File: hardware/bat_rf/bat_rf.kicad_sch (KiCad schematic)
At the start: 54 parts, among them J1 USB_C_Receptacle_PowerOnly_6P, J2 Conn_01x02, J3 burningPort, Q1 NMOS, SW1 SW_DPDT_x2, SW2 RESET, U1 TPS5430DDA, U2 AMS1117, U3 ESP8684-WROOM-02UC, U4 CS5090E

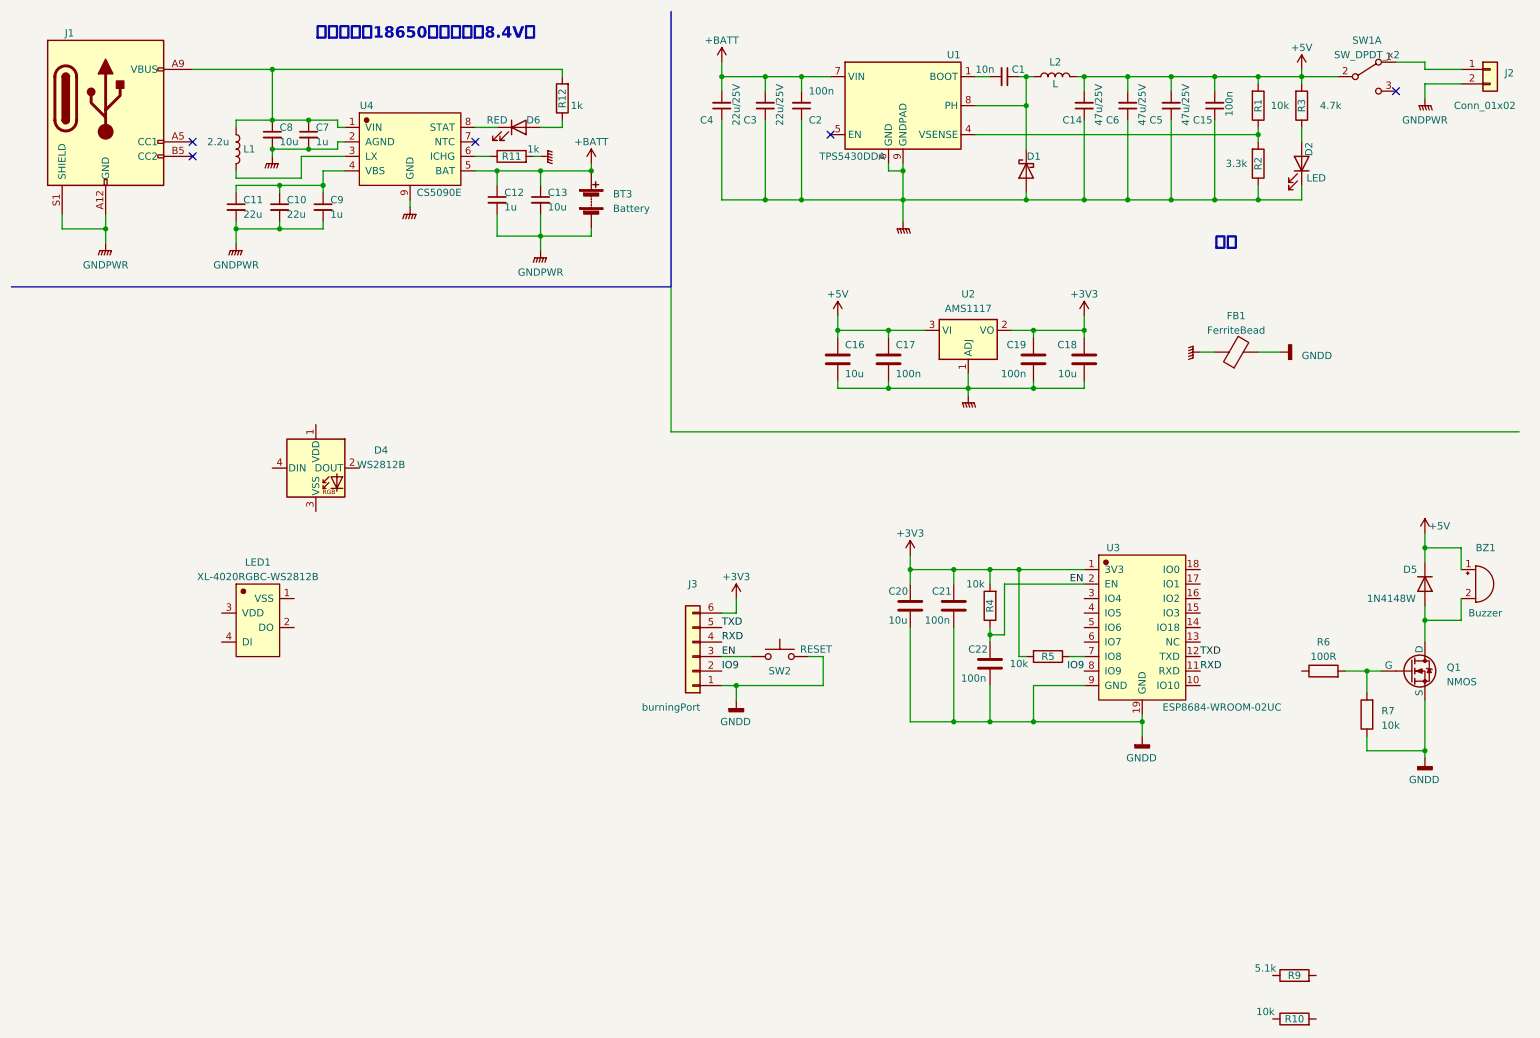
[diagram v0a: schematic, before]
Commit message: hardware update
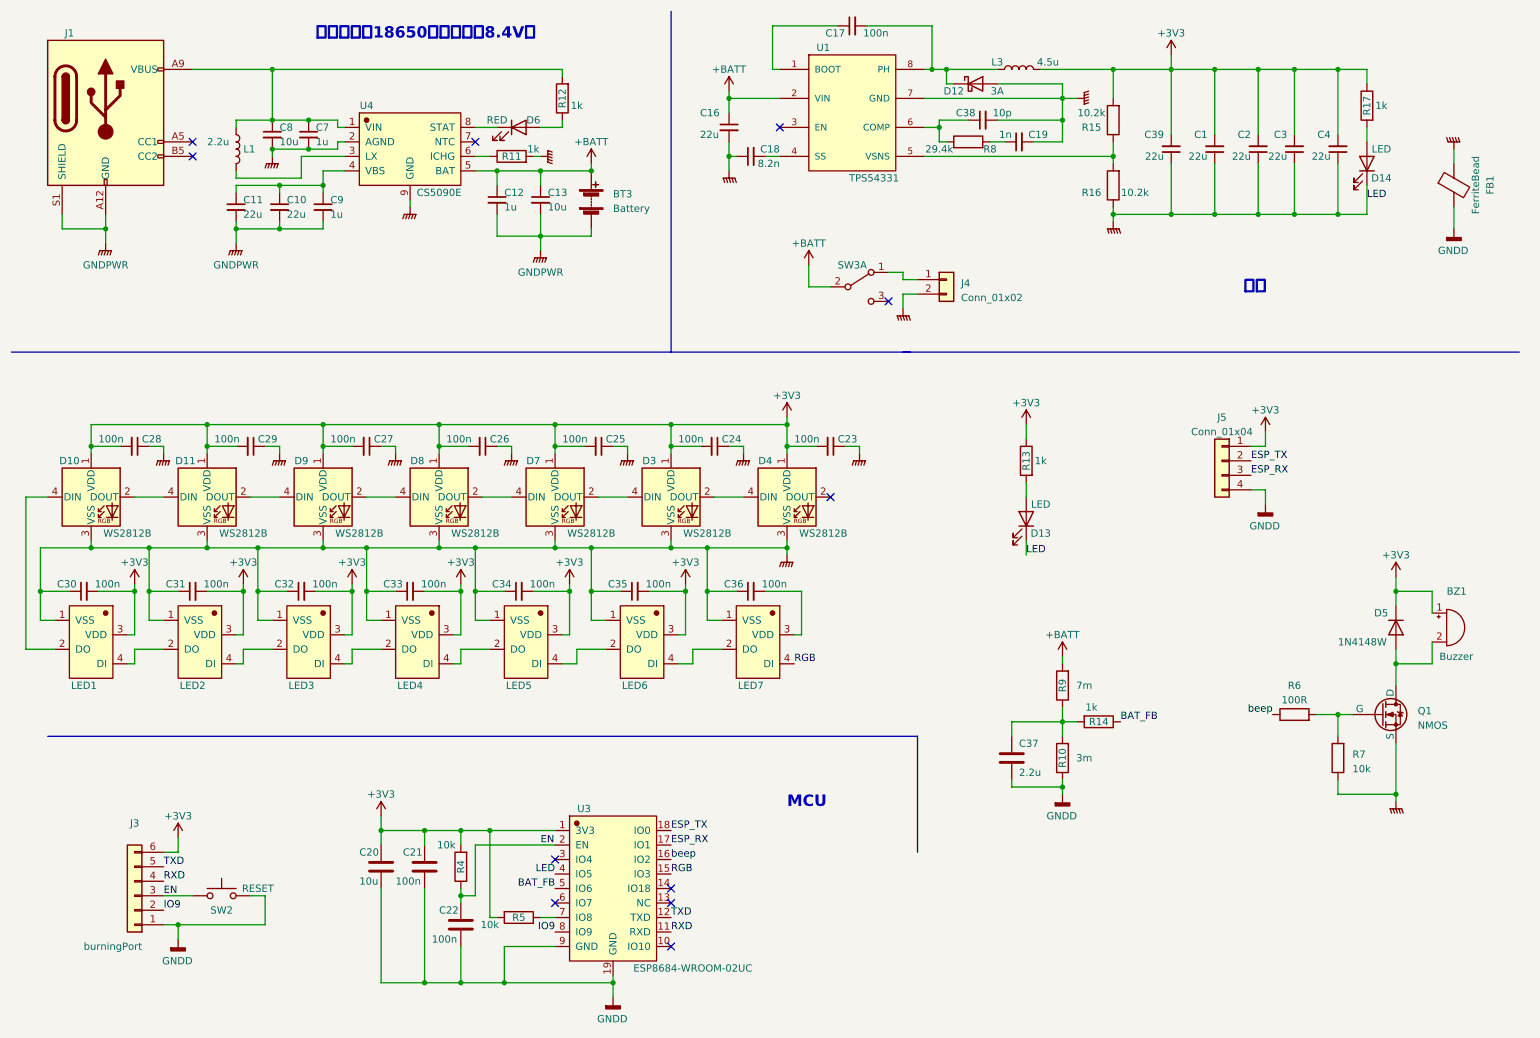
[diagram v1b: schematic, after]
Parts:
- removed C14, C5, C6: 47u/25V, symbol Device:C_Small
- removed C15: 100n, symbol Device:C_Small
- removed C16, C18: 10u, symbol Device:C
- removed C17, C19: 100n, symbol Device:C
- removed D1: 1N5819WS, Diode_SMD:D_SOD-323, symbol Diode:1N5819WS
- removed D2: LED, LED_SMD:LED_0603_1608Metric_Pad1.05x0.95mm_HandSolder, symbol Device:LED
- removed J2: Conn_01x02, symbol Connector_Generic:Conn_01x02
- removed L2: L, symbol Device:L
- removed R1: 10k, Resistor_SMD:R_0603_1608Metric_Pad0.98x0.95mm_HandSolder, symbol Device:R
- removed R2: 3.3k, Resistor_SMD:R_0603_1608Metric_Pad0.98x0.95mm_HandSolder, symbol Device:R
- removed R3: 4.7k, Resistor_SMD:R_0603_1608Metric_Pad0.98x0.95mm_HandSolder, symbol Device:R
- removed SW1: SW_DPDT_x2, symbol Switch:SW_DPDT_x2
- removed U1: TPS5430DDA, Package_SO:TI_SO-PowerPAD-8_ThermalVias, symbol Regulator_Switching:TPS5430DDA
- removed U2: AMS1117, Package_TO_SOT_SMD:SOT-223-3_TabPin2, symbol Regulator_Linear:AMS1117
- added C16, C39: 22u, Capacitor_SMD:C_0805_2012Metric_Pad1.18x1.45mm_HandSolder, symbol Device:C_Small
- added C17, C23, C24, C25, C26, C27, C28, C29, C30, C31, C32, C33, C34, C35, C36: 100n, Capacitor_SMD:C_0603_1608Metric_Pad1.08x0.95mm_HandSolder, symbol Device:C_Small
- added C18: 8.2n, Capacitor_SMD:C_0603_1608Metric_Pad1.08x0.95mm_HandSolder, symbol Device:C_Small
- added C19: 1n, Capacitor_SMD:C_0603_1608Metric_Pad1.08x0.95mm_HandSolder, symbol Device:C_Small
- added C37: 2.2u, Capacitor_SMD:C_0603_1608Metric_Pad1.08x0.95mm_HandSolder, symbol Device:C
- added C38: 10p, Capacitor_SMD:C_0603_1608Metric_Pad1.08x0.95mm_HandSolder, symbol Device:C_Small
- added D10, D11, D3, D7, D8, D9: WS2812B, LED_SMD:LED_WS2812B_PLCC4_5.0x5.0mm_P3.2mm, symbol LED:WS2812B
- added D12: 3A, Diode_SMD:D_MELF, symbol Diode:1N5711UR
- added D13, D14: LED, LED_SMD:LED_0603_1608Metric_Pad1.05x0.95mm_HandSolder, symbol Device:LED
- added J4: Conn_01x02, bat_rf:CONN-TH_XT30U-M, symbol Connector_Generic:Conn_01x02
- added J5: Conn_01x04, Connector_PinHeader_2.54mm:PinHeader_1x04_P2.54mm_Vertical_SMD_Pin1Left, symbol Connector_Generic:Conn_01x04
- added L3: 4.5u, bat_rf:IND-SMD_L7.0-W6.6_0630CDMCCDS, symbol Device:L
- added LED2, LED3, LED4, LED5, LED6, LED7: XL-4020RGBC-WS2812B, bat_rf:LED-SMD_4P-L4.0-W1.7_M4020-03003-RGB-862-001, symbol bat_rf:XL-4020RGBC-WS2812B
- added R13, R14, R17: 1k, Resistor_SMD:R_0603_1608Metric_Pad0.98x0.95mm_HandSolder, symbol Device:R
- added R15, R16: 10.2k, Resistor_SMD:R_0603_1608Metric_Pad0.98x0.95mm_HandSolder, symbol Device:R
- added R8: 29.4k, Resistor_SMD:R_0603_1608Metric_Pad0.98x0.95mm_HandSolder, symbol Device:R
- added SW3: SW_DPDT_x2, bat_rf:SW-TH_3P-SS12D06-1, symbol Switch:SW_DPDT_x2
- added U1: TPS54331, bat_rf:SOP8-PAD, symbol bat_rf:TPS54331
- BT3: footprint (none) -> bat_rf:BAT-SMD_BH-18650-B1BA007
- BZ1: footprint (none) -> Buzzer_Beeper:Buzzer_12x9.5RM7.6
- C1: value 10n -> 22u; footprint (none) -> Capacitor_SMD:C_0805_2012Metric_Pad1.18x1.45mm_HandSolder
- C10, C11, C13, C20, C8: footprint (none) -> Capacitor_SMD:C_0805_2012Metric_Pad1.18x1.45mm_HandSolder
- C12, C21, C22, C7, C9, FB1: footprint (none) -> Capacitor_SMD:C_0603_1608Metric_Pad1.08x0.95mm_HandSolder
- C2: value 100n -> 22u; footprint (none) -> Capacitor_SMD:C_0805_2012Metric_Pad1.18x1.45mm_HandSolder
- C3, C4: value 22u/25V -> 22u; footprint (none) -> Capacitor_SMD:C_0805_2012Metric_Pad1.18x1.45mm_HandSolder
- J3: footprint (none) -> Connector_PinHeader_2.54mm:PinHeader_1x06_P2.54mm_Vertical
- L1: footprint (none) -> bat_rf:IND-SMD_L7.0-W6.6_0630CDMCCDS
- LED1: footprint kicad_lceda:LED-SMD_4P-L4.0-W1.7_M4020-03003-RGB-862-001 -> bat_rf:LED-SMD_4P-L4.0-W1.7_M4020-03003-RGB-862-001
- Q1: footprint (none) -> Package_TO_SOT_SMD:SOT-23
- R10: value 10k -> 3m
- R6, R7: footprint (none) -> Resistor_SMD:R_0603_1608Metric_Pad0.98x0.95mm_HandSolder
- R9: value 5.1k -> 7m
- SW2: footprint (none) -> Button_Switch_SMD:SW_SPST_B3U-1000P
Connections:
- net +5V is gone; now on net +3V3: BZ1.1 (-), D5.1 (K)
- net +3V3: now also C1.2, C2.2, C3.2, C4.2, D4.1 (VDD), LED1.3 (VDD), C23.2, C24.2, C25.2, C26.2, C27.2, C28.2, C29.2, C30.2, C31.2, C32.2, C33.2, C34.2, C35.2, C39.2, D10.1 (VDD), D11.1 (VDD), D3.1 (VDD), D7.1 (VDD), D8.1 (VDD), D9.1 (VDD), J5.1 (Pin_1), L3.2, LED2.3 (VDD), LED3.3 (VDD), LED4.3 (VDD), LED5.3 (VDD), LED6.3 (VDD), R13.1, R15.2, R17.1
- net +BATT: now also R9.2, C16.1, SW3.2 (B), U1.2 (VIN); no longer C2.2, C3.2, C4.2
- net GNDD: now also R10.1, C37.2, J5.4 (Pin_4); no longer Q1.3 (S), R7.1
- net GNDPWR: now also C1.1, D4.3 (VSS), LED1.1 (VSS), Q1.3 (S), R7.1, U3.4 (IO5), C16.2, C18.1, C19.2, C23.1, C24.1, C25.1, C26.1, C27.1, C28.1, C29.1, C30.1, C31.1, C32.1, C33.1, C34.1, C35.1, C36.1, C38.2, C39.1, D10.3 (VSS), D11.3 (VSS), D12.2 (A), D13.1 (K), D14.1 (K), D3.3 (VSS), D7.3 (VSS), D8.3 (VSS), D9.3 (VSS), J4.2 (Pin_2), LED2.1 (VSS), LED3.1 (VSS), LED4.1 (VSS), LED5.1 (VSS), LED6.1 (VSS), LED7.1 (VSS), R16.1, U1.7 (GND)
- net at R9.1: now also R10.2, C37.1, R14.2
- net at LED1.2 (DO): now also D10.4 (DIN)
- net at LED1.4 (DI): now also LED2.2 (DO)
- net beep: now reaches R6.1
- net beep: now also U3.16 (IO2)
- net at D4.4 (DIN): now also D3.2 (DOUT)
- net RGB: now reaches U3.15 (IO3)
- net RGB: now also LED7.4 (DI)
- net ESP_RX: now reaches U3.17 (IO1)
- net ESP_RX: now also J5.3 (Pin_3)
- net ESP_TX: now reaches U3.18 (IO0)
- net ESP_TX: now also J5.2 (Pin_2)
- net BAT_FB: now reaches U3.5 (IO6)
- net BAT_FB: now also R14.1
- new net: C17.2, D12.1 (K), L3.1, U1.8 (PH)
- new net: C19.1, R8.2
- new net: D13.2 (A), R13.2
- new net: C38.1, R8.1, U1.6 (COMP)
- new net: D14.2 (A), R17.2
- new net: C36.2, LED7.3 (VDD)
- new net: R15.1, R16.2, U1.5 (VSNS)
- new net: J4.1 (Pin_1), SW3.1 (A)
- new net: LED5.4 (DI), LED6.2 (DO)
- new net: LED6.4 (DI), LED7.2 (DO)
- new net: C17.1, U1.1 (BOOT)
- new net: C18.2, U1.4 (SS)
- new net: D3.4 (DIN), D7.2 (DOUT)
- new net: D10.2 (DOUT), D11.4 (DIN)
- new net: D8.4 (DIN), D9.2 (DOUT)
- new net: D11.2 (DOUT), D9.4 (DIN)
- new net: LED4.4 (DI), LED5.2 (DO)
- new net: LED2.4 (DI), LED3.2 (DO)
- new net: LED3.4 (DI), LED4.2 (DO)
- new net: D7.4 (DIN), D8.2 (DOUT)
- no-connect marks 5 -> 11
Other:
- note added: "MCU"
- moved on the sheet: BZ1, C20, C21, C22, D4, D5, FB1, J3, LED1, Q1, R10, R4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
